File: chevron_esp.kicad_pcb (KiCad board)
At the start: 2 copper layers, 160 x 80 mm, 24 parts, among them J1 282837-4, K1 SRD-05VDC-SL-C, K2 SRD-05VDC-SL-C, K3 SRD-05VDC-SL-C, P1 282837-2, Q1 PN2222A, Q2 PN2222A, Q3 PN2222A, SW1 1825057-2, U1 ESP32-DEVKIT-V1, U2 RA-02_LORA

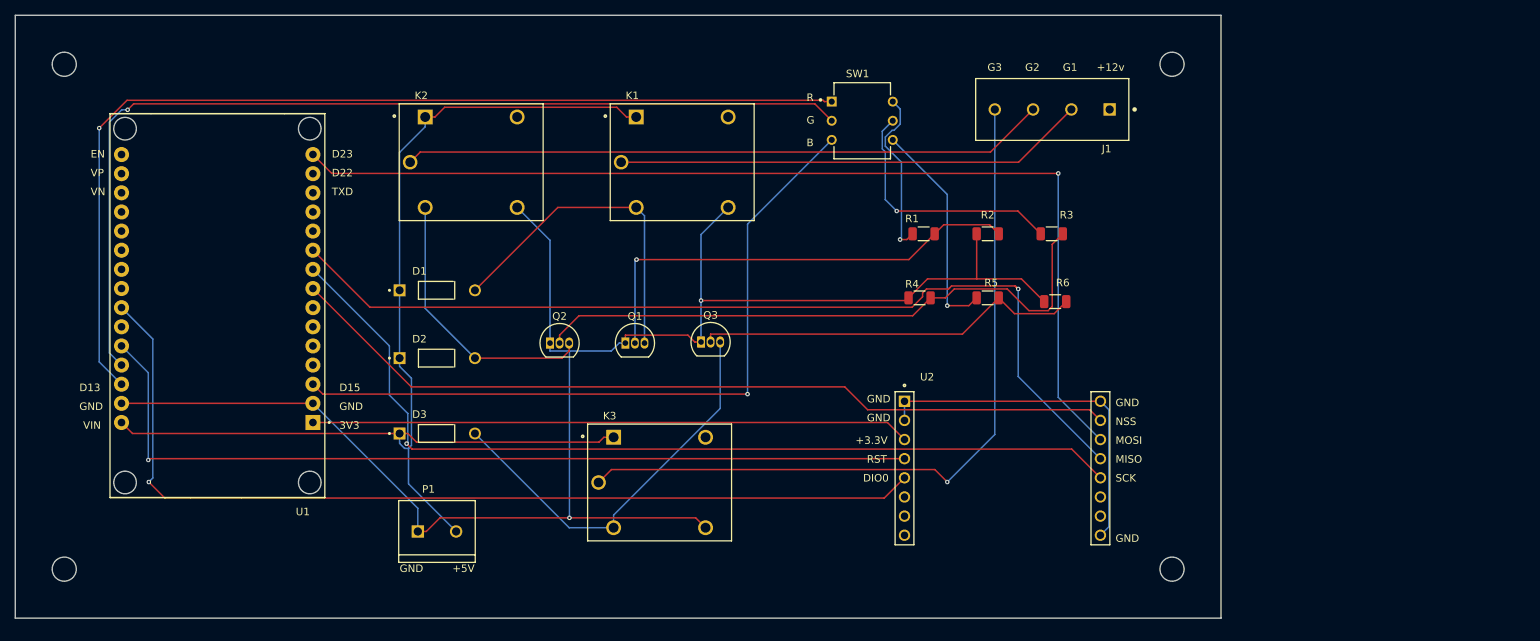
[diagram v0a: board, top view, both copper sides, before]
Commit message: chevron esp v1.2
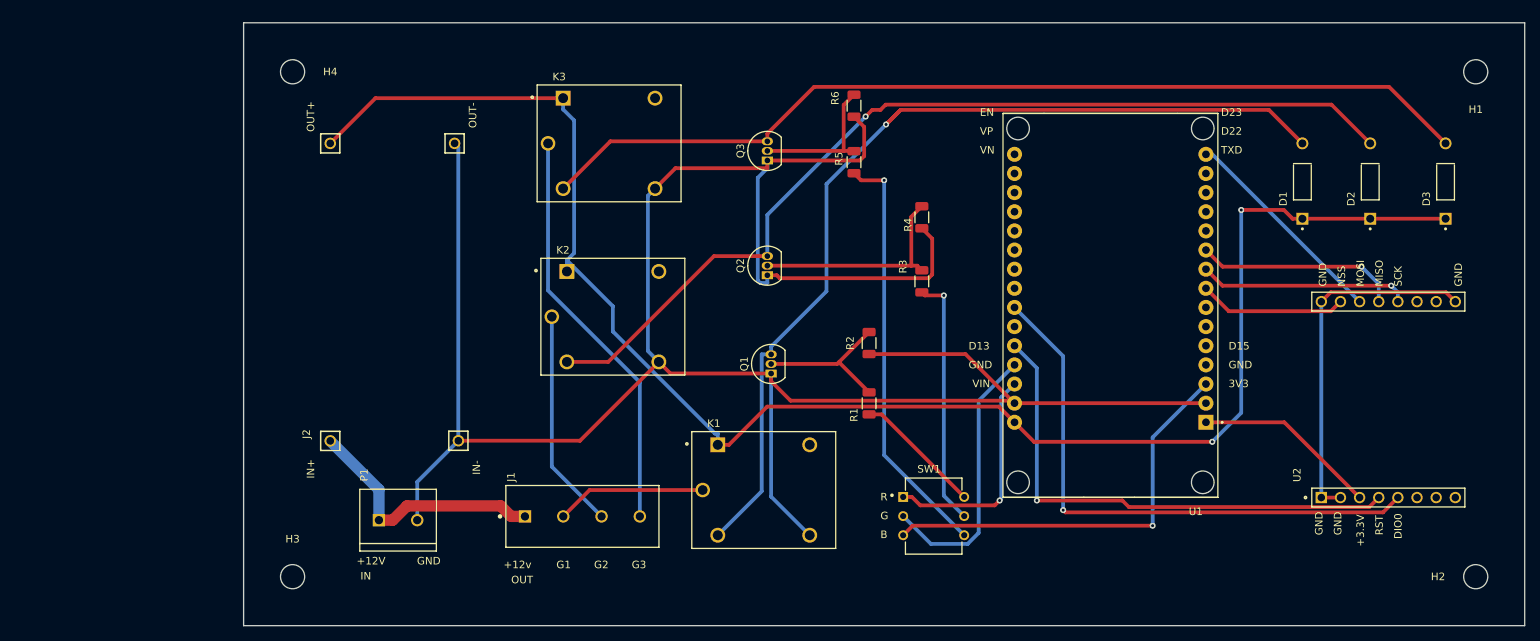
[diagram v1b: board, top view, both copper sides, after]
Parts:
- removed ~ (x4): MountingHole_3.2mm_M3, MountingHole:MountingHole_3.2mm_M3
- added H1: MountingHole_3.2mm_M3, MountingHole:MountingHole_3.2mm_M3, F.Cu at (228.8, 62.5)
- added H2: MountingHole_3.2mm_M3, MountingHole:MountingHole_3.2mm_M3, F.Cu at (228.8, 129.5)
- added H3: MountingHole_3.2mm_M3, MountingHole:MountingHole_3.2mm_M3, F.Cu at (71.8, 129.5)
- added H4: MountingHole_3.2mm_M3, MountingHole:MountingHole_3.2mm_M3, F.Cu at (71.8, 62.5)
- added J2: MTSW-101-09-G-S-104x4, MTSW-101-09-G-S-104:SAMTEC_MTSW-101-09-G-S-104x4, F.Cu at (76.8, 111.5)
- moved D3 137.9 mm to (224.8, 77.0), turned to 90 degrees
- moved D2 126.0 mm to (214.8, 77.0), turned to 90 degrees
- moved U1 118.5 mm to (180.3, 93.5)
- moved D1 115.7 mm to (205.8, 77.0), turned to 90 degrees
- moved J1 94.5 mm to (102.6, 121.5), turned to 0 degrees
- moved U2 62.1 mm to (219.1, 115.0), turned to 90 degrees
- moved SW1 53.3 mm to (152.8, 118.9)
- moved K3 45.5 mm to (113.8, 72.0)
- moved K1 44.8 mm to (134.3, 118.0)
- moved R6 37.3 mm to (146.3, 67.0), turned to 90 degrees
- moved Q2 30.2 mm to (134.8, 89.5), turned to 90 degrees
- moved K2 27.8 mm to (114.3, 95.0)
- moved Q3 25.6 mm to (134.8, 74.3), turned to 90 degrees
- moved R5 25.3 mm to (146.3, 74.5), turned to 90 degrees
- moved R1 23.6 mm to (148.3, 106.5), turned to 90 degrees
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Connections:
- J1 pad 1: unconnected-(J1-Pad1) -> +12V
- P1 pad 1: GND -> +12V
- P1 pad 2: +5V -> GND
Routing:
- net Net-(U1-D23): track 137.6 -> 28.5 mm, vias 1 -> 0
- net Net-(U1-D13): track 134.0 -> 29.8 mm
- net Net-(U1-D19): track 126.8 -> 27.1 mm
- net Net-(U1-D18): track 122.4 -> 28.0 mm
- net Net-(U1-D12): track 130.7 -> 36.4 mm, vias 1 -> 0
- net Net-(U1-D5): track 111.7 -> 19.6 mm
- net Net-(Q2-C): track 36.7 -> 126.1 mm, vias 0 -> 1
- net GND: track 226.4 -> 312.2 mm, vias 2 -> 0
- net Net-(Q1-C): track 44.4 -> 124.9 mm, vias 0 -> 1
- net Net-(Q3-C): track 54.1 -> 126.4 mm
- net +5V: track 158.3 -> 220.0 mm, vias 0 -> 2
- net Net-(J1-Pad3): track 85.6 -> 29.2 mm
- net Net-(U1-3V3): track 79.4 -> 24.5 mm
- net Net-(U1-D26): track 127.3 -> 74.9 mm
- net Net-(Q2-B): track 80.6 -> 29.2 mm
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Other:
- board size 160 x 80 mm -> 170 x 80 mm
- board text added: "+12V"
- board text added: "IN"
- board text added: "OUT"
- board text removed: "+5V"

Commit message: v1 ok
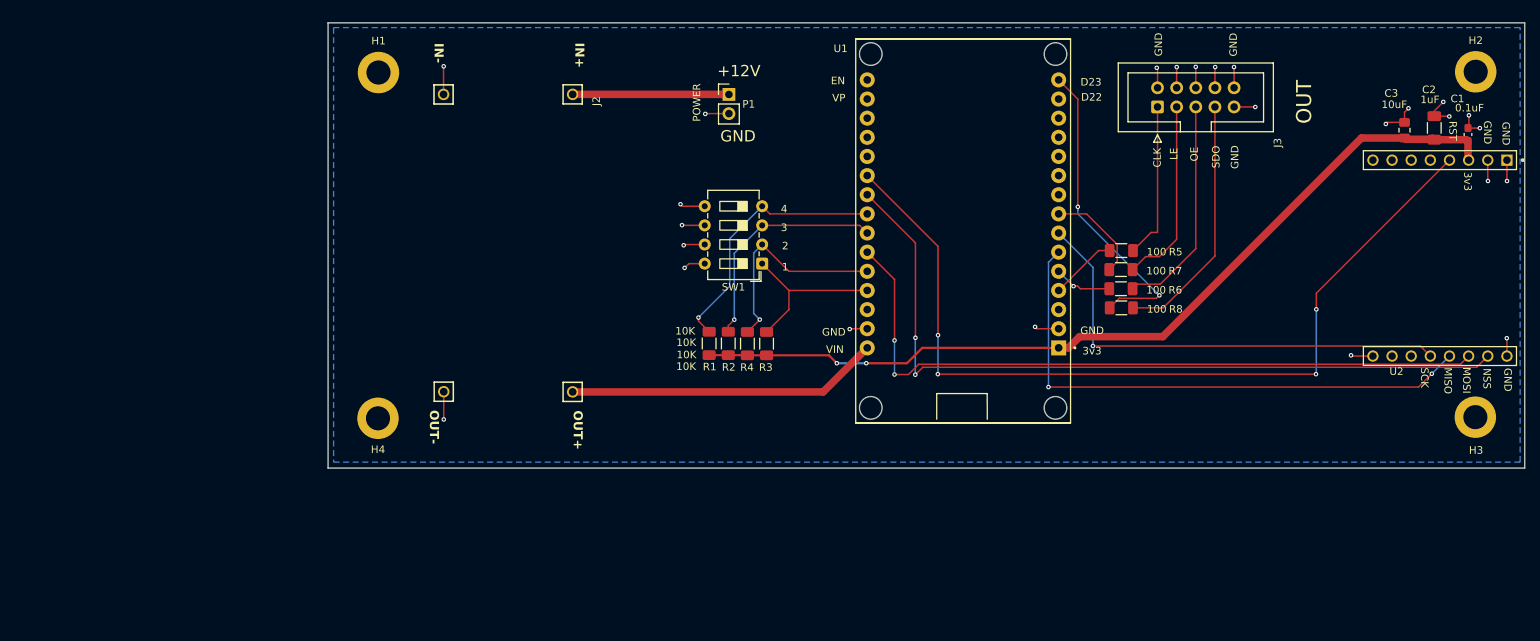
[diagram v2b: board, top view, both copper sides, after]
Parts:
- removed D1, D2, D3: 1N4007-T, 1N4007-T:DIOAD780W78L463D236
- removed J1: 282837-4, 282837-4:TE_282837-4
- removed K1, K2, K3: SRD-05VDC-SL-C, SRD-05VDC-SL-C:RELAY_SRD-05VDC-SL-C
- removed Q1, Q2, Q3: PN2222A, Package_TO_SOT_THT:TO-92_Inline
- added C1: 0.1uF, Capacitor_SMD:C_0603_1608Metric_Pad1.08x0.95mm_HandSolder, F.Cu at (227.8, 70.8)
- added C2: 1uF, Capacitor_SMD:C_1206_3216Metric_Pad1.33x1.80mm_HandSolder, F.Cu at (223.3, 70.0)
- added C3: 10uF, Capacitor_SMD:C_0805_2012Metric_Pad1.18x1.45mm_HandSolder, F.Cu at (219.3, 70.2)
- added J3: Conn_02x05_Counter_Clockwise, Connector_IDC:IDC-Header_2x05_P2.54mm_Vertical, F.Cu at (186.6, 67.2)
- added R7: 100, Resistor_SMD:R_1206_3216Metric_Pad1.30x1.75mm_HandSolder, F.Cu at (181.7, 88.8)
- added R8: 100, Resistor_SMD:R_1206_3216Metric_Pad1.30x1.75mm_HandSolder, F.Cu at (181.8, 93.8)
- H1: renamed from H4; value MountingHole_3.2mm_M3 -> 3.2mm_M3_TH; footprint MountingHole:MountingHole_3.2mm_M3 -> Mounting Hole:3.2mm_M3_TH
- H2: renamed from H1; value MountingHole_3.2mm_M3 -> 3.2mm_M3_TH; footprint MountingHole:MountingHole_3.2mm_M3 -> Mounting Hole:3.2mm_M3_TH
- H3: renamed from H2; value MountingHole_3.2mm_M3 -> 3.2mm_M3_TH; footprint MountingHole:MountingHole_3.2mm_M3 -> Mounting Hole:3.2mm_M3_TH
- H4: renamed from H3; value MountingHole_3.2mm_M3 -> 3.2mm_M3_TH; footprint MountingHole:MountingHole_3.2mm_M3 -> Mounting Hole:3.2mm_M3_TH
- P1: footprint 282837-2:TE_282837-2 -> Connector_PinHeader_2.54mm:PinHeader_1x02_P2.54mm_Vertical
- R1, R3: value 330 -> 10K; footprint Resistor_SMD:R_1206_3216Metric -> Resistor_SMD:R_1206_3216Metric_Pad1.30x1.75mm_HandSolder
- R2, R4: value 10k -> 10K; footprint Resistor_SMD:R_1206_3216Metric -> Resistor_SMD:R_1206_3216Metric_Pad1.30x1.75mm_HandSolder
- R5: value 330 -> 100; footprint Resistor_SMD:R_1206_3216Metric -> Resistor_SMD:R_1206_3216Metric_Pad1.30x1.75mm_HandSolder
- R6: value 10k -> 100; footprint Resistor_SMD:R_1206_3216Metric -> Resistor_SMD:R_1206_3216Metric_Pad1.30x1.75mm_HandSolder
- SW1: value 1825057-2 -> SW_DIP_x04; footprint 1825057-2:DIP810W60P254L1010H480Q6 -> Button_Switch_THT:SW_DIP_SPSTx04_Slide_6.7x11.72mm_W7.62mm_P2.54mm_LowProfile
- moved P1 71.5 mm to (129.7, 65.5)
- moved R6 43.0 mm to (181.7, 91.3), turned to 0 degrees
- moved J2 39.6 mm to (103.0, 81.7), turned to -90 degrees
- moved R5 37.4 mm to (181.8, 86.2), turned to 0 degrees
- moved U2 36.9 mm to (222.2, 78.2), turned to -90 degrees
- moved SW1 36.2 mm to (134.1, 88.0), turned to 180 degrees
- moved R4 28.6 mm to (132.2, 98.6), turned to -90 degrees
- moved H4 23.9 mm to (83.1, 108.5)
- moved R1 22.7 mm to (127.1, 98.6), turned to -90 degrees
- moved R3 22.2 mm to (134.7, 98.6), turned to -90 degrees
- moved U1 21.9 mm to (160.8, 83.6)
- moved H3 21.2 mm to (228.8, 108.3)
- moved R2 18.7 mm to (129.6, 98.6), turned to -90 degrees
- moved H1 11.4 mm to (83.2, 62.6)
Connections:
- H1 pad : (no net) -> GND
- H2 pad : (no net) -> GND
- H3 pad : (no net) -> GND
- H4 pad : (no net) -> GND
- R1 pad 1: Net-(R1-Pad1) -> Net-(U1-D25)
- R1 pad 2: Net-(Q1-B) -> VDD_3V3
- R2 pad 1: GND -> Net-(U1-D26)
- R2 pad 2: Net-(Q1-B) -> VDD_3V3
- R3 pad 1: Net-(R3-Pad1) -> Net-(U1-D12)
- R3 pad 2: Net-(Q2-B) -> VDD_3V3
- R4 pad 1: GND -> Net-(U1-D14)
- R4 pad 2: Net-(Q2-B) -> VDD_3V3
- R5 pad 1: Net-(R5-Pad1) -> Net-(U1-D2)
- R5 pad 2: Net-(Q3-B) -> CLK
- R6 pad 1: GND -> Net-(U1-D4)
- R6 pad 2: Net-(Q3-B) -> OE
- SW1 pad 1: Net-(U1-D13) -> Net-(U1-D12)
- SW1 pad 2: Net-(U1-D12) -> Net-(U1-D14)
- SW1 pad 3: Net-(U1-D15) -> Net-(U1-D26)
- SW1 pad 4: Net-(R5-Pad1) -> Net-(U1-D25)
- SW1 pad 5: Net-(R3-Pad1) -> GND
- SW1 pad 6: Net-(R1-Pad1) -> GND
- U1 pad 1: Net-(U1-3V3) -> VDD_3V3
- U1 pad 10: Net-(U1-D19) -> unconnected-(U1-D19-Pad10)
- U1 pad 21: unconnected-(U1-D32-Pad21) -> Net-(U1-D32)
- U1 pad 22: unconnected-(U1-D33-Pad22) -> Net-(U1-D33)
- U1 pad 23: unconnected-(U1-D25-Pad23) -> Net-(U1-D25)
- U1 pad 25: unconnected-(U1-D27-Pad25) -> Net-(U1-D27)
- U1 pad 28: Net-(U1-D13) -> unconnected-(U1-D13-Pad28)
- U1 pad 3: Net-(U1-D15) -> unconnected-(U1-D15-Pad3)
- U1 pad 4: unconnected-(U1-D2-Pad4) -> Net-(U1-D2)
- U1 pad 5: unconnected-(U1-D4-Pad5) -> Net-(U1-D4)
- U1 pad 6: unconnected-(U1-RX2-Pad6) -> Net-(U1-RX2)
- U1 pad 7: unconnected-(U1-TX2-Pad7) -> Net-(U1-TX2)
- U1 pad 9: Net-(U1-D18) -> unconnected-(U1-D18-Pad9)
- U2 pad 1: Net-(U2-GND-Pad1) -> GND
- U2 pad 12: Net-(U1-D18) -> Net-(U1-TX2)
- U2 pad 13: Net-(U1-D19) -> Net-(U1-RX2)
- U2 pad 14: Net-(U1-D23) -> Net-(U1-D27)
- U2 pad 15: Net-(U1-D5) -> Net-(U1-D33)
- U2 pad 16: Net-(U2-GND-Pad1) -> GND
- U2 pad 2: Net-(U2-GND-Pad1) -> GND
- U2 pad 3: Net-(U1-3V3) -> VDD_3V3
- U2 pad 4: Net-(U1-D14) -> Net-(U1-D32)
- U2 pad 5: Net-(U1-D26) -> unconnected-(U2-DI00-Pad5)
- U2 pad 9: Net-(U2-GND-Pad1) -> GND
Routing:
- net GND: track 312.2 -> 67.9 mm, vias 0 -> 25
- net +5V: track 220.0 -> 41.5 mm, vias 2 -> 0
- net Net-(Q3-C): track 126.4 -> 0.00 mm
- net Net-(Q2-C): track 126.1 -> 0.00 mm, vias 1 -> 0
- net Net-(Q1-C): track 124.9 -> 0.00 mm, vias 1 -> 0
- net Net-(U1-D32): track 0.00 -> 116.2 mm, vias 0 -> 4
- net VDD_3V3: track 0.00 -> 115.7 mm, vias 0 -> 2
- net Net-(U1-D33): track 0.00 -> 104.5 mm, vias 0 -> 2
- net Net-(U1-D27): track 0.00 -> 96.0 mm, vias 0 -> 2
- net Net-(U1-RX2): track 0.00 -> 73.4 mm, vias 0 -> 2
- net Net-(U1-TX2): track 0.00 -> 63.2 mm, vias 0 -> 1
- net Net-(R5-Pad1): track 55.9 -> 0.00 mm, vias 1 -> 0
- net Net-(U1-D15): track 55.4 -> 0.00 mm, vias 1 -> 0
- net Net-(J1-Pad4): track 54.5 -> 0.00 mm
- net Net-(U2-GND-Pad1): track 47.4 -> 0.00 mm
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- added copper zone on B.Cu, net GND
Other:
- board size 170 x 80 mm -> 158.8 x 59.1 mm
- board text added: "1"
- board text added: "2"
- board text added: "3"
- board text added: "3v3"
- board text added: "4"
- board text added: "CLK"
- board text added: "LE"
- board text added: "OE"
- board text added: "POWER"
- board text added: "SDO"
- board text removed: "+12v"
- board text removed: "+3.3V"
- board text removed: "3V3"
- board text removed: "B"
- board text removed: "D13"
- board text removed: "D15"
- board text removed: "DIO0"
- board text removed: "G"
- board text removed: "G1"
- board text removed: "G2"
- board text removed: "G3"
- board text removed: "IN"
- board text removed: "R"
- board text removed: "TXD"
- board text removed: "VN"
